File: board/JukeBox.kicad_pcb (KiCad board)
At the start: 2 copper layers, 88 x 88 mm, 68 parts, among them J1 USB_C_Receptacle_USB2.0, J2 Conn_01x03, J3 Conn_01x04, SW1 SW_SPST, SW10 SW_SPST, SW11 SW_SPST, SW12 SW_SPST, SW2 SW_SPST, SW3 SW_SPST, SW4 SW_SPST, SW5 SW_SPST, SW6 SW_SPST, SW7 SW_SPST, SW8 SW_SPST, SW9 SW_SPST, U1 NCP1117-3.3_SOT223, U2 W25Q128JVS, U3 RP2040, Y1 ABLS-12.000MHZ-B4-T

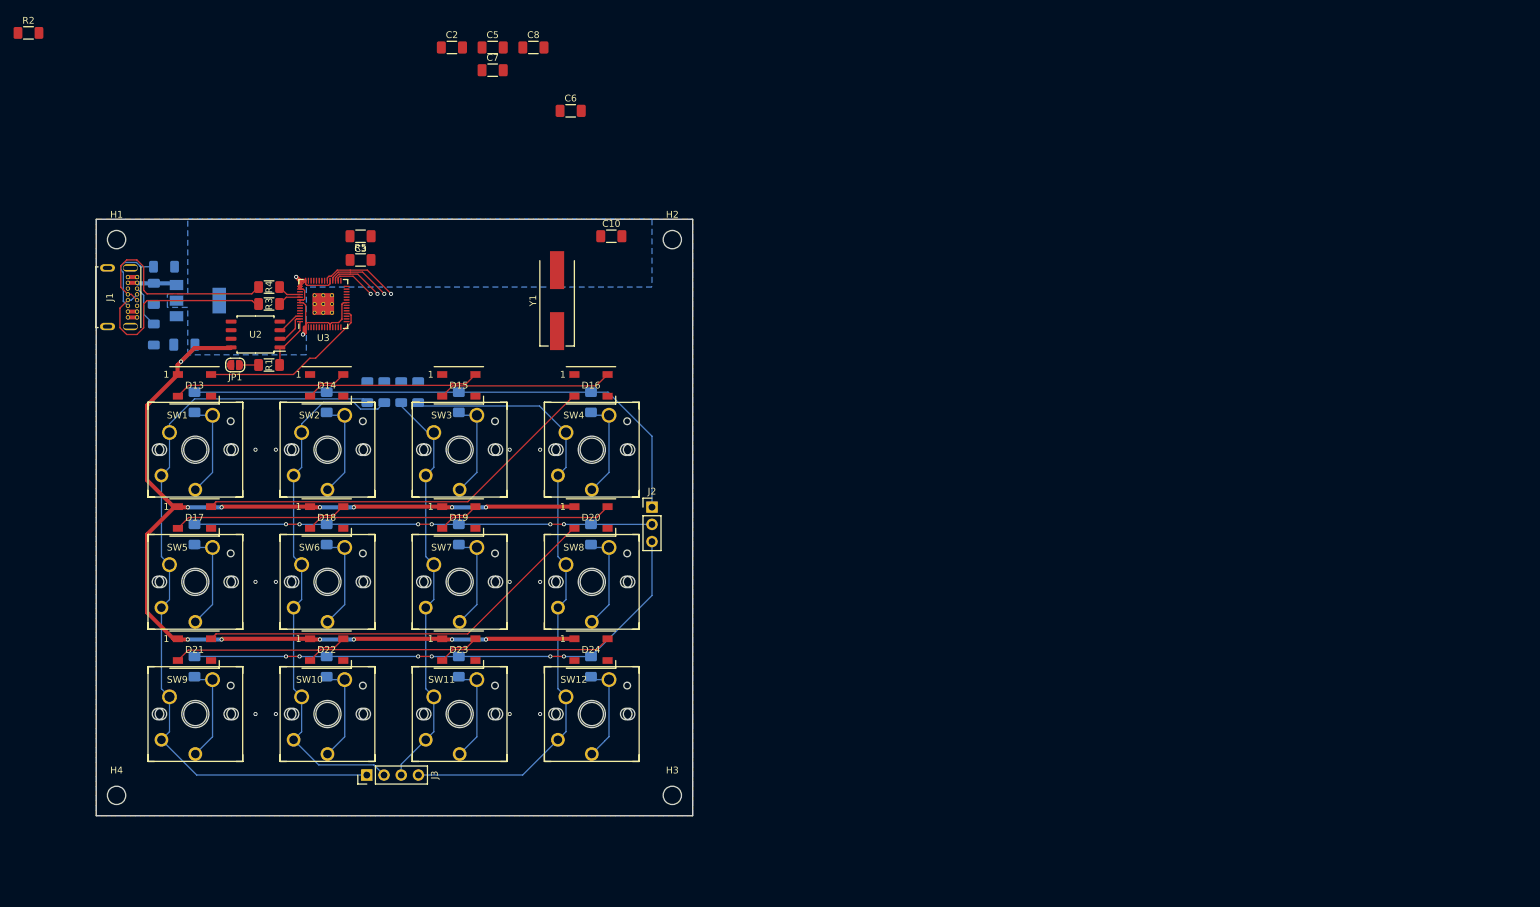
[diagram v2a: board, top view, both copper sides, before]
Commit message: second pass pcb
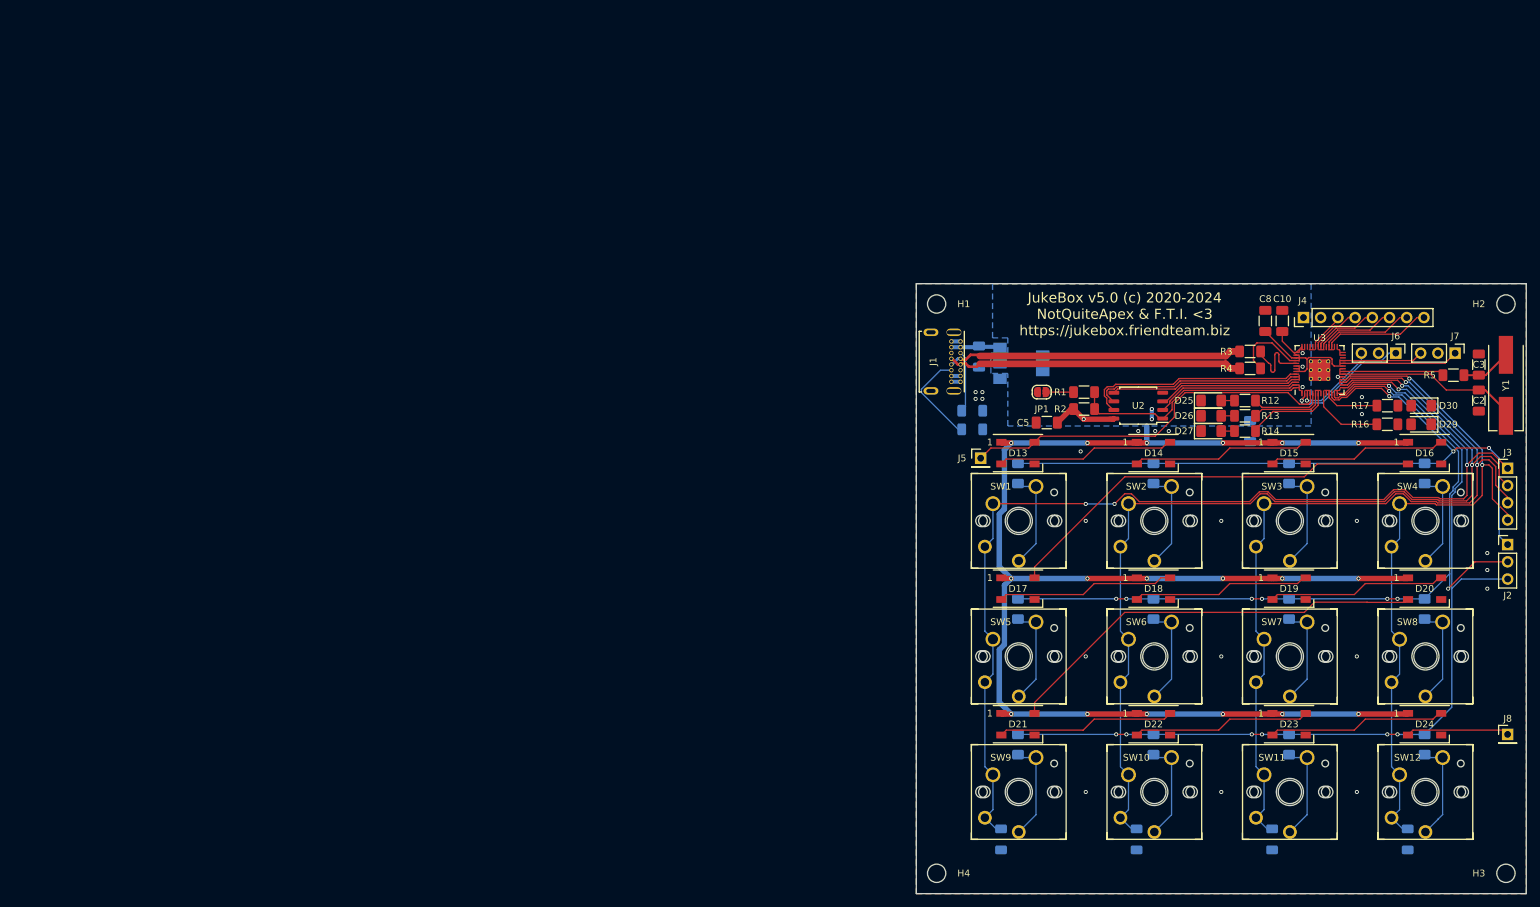
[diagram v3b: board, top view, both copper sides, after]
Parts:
- removed C6, C7: 100n, Capacitor_SMD:C_1206_3216Metric_Pad1.33x1.80mm_HandSolder
- added D25: LED, Diode_SMD:D_1206_3216Metric_Pad1.42x1.75mm_HandSolder, F.Cu at (211.1, 72.2)
- added D26: LED, Diode_SMD:D_1206_3216Metric_Pad1.42x1.75mm_HandSolder, F.Cu at (211.1, 74.5)
- added D27: LED, Diode_SMD:D_1206_3216Metric_Pad1.42x1.75mm_HandSolder, F.Cu at (211.1, 76.8)
- added D29: LED, Diode_SMD:D_1206_3216Metric_Pad1.42x1.75mm_HandSolder, F.Cu at (242.1, 75.8)
- added D30: LED, Diode_SMD:D_1206_3216Metric_Pad1.42x1.75mm_HandSolder, F.Cu at (242.1, 73.0)
- added J4: Conn_01x08, Connector_PinHeader_2.54mm:PinHeader_1x08_P2.54mm_Vertical, F.Cu at (224.7, 60.0)
- added J5: Conn_01x01, Connector_PinHeader_2.54mm:PinHeader_1x01_P2.54mm_Vertical, F.Cu at (177.1, 80.8)
- added J6: Conn_01x03, Connector_PinHeader_2.54mm:PinHeader_1x03_P2.54mm_Vertical, F.Cu at (238.3, 65.2)
- added J7: Conn_01x03, Connector_PinHeader_2.54mm:PinHeader_1x03_P2.54mm_Vertical, F.Cu at (247.1, 65.2)
- added J8: Conn_01x01, Connector_PinHeader_2.54mm:PinHeader_1x01_P2.54mm_Vertical, F.Cu at (254.8, 121.5)
- added R10: 10k, Resistor_SMD:R_1206_3216Metric_Pad1.30x1.75mm_HandSolder, B.Cu at (220.1, 137.0)
- added R16: 200, Resistor_SMD:R_1206_3216Metric_Pad1.30x1.75mm_HandSolder, F.Cu at (237.1, 75.8)
- added R17: 200, Resistor_SMD:R_1206_3216Metric_Pad1.30x1.75mm_HandSolder, F.Cu at (237.1, 73.0)
- added R8: 10k, Resistor_SMD:R_1206_3216Metric_Pad1.30x1.75mm_HandSolder, B.Cu at (180.1, 137.0)
- added R9: 10k, Resistor_SMD:R_1206_3216Metric_Pad1.30x1.75mm_HandSolder, B.Cu at (200.1, 137.0)
- R12, R13, R14: value 10k -> 200; moved to F.Cu
- moved J3 174.3 mm to (254.8, 82.2), turned to 0 degrees
- moved R11 167.1 mm to (240.1, 137.0), turned to 90 degrees
- moved C3 166.1 mm to (250.6, 66.9), turned to 90 degrees
- moved R2 165.3 mm to (192.3, 73.5)
- moved R5 162.1 mm to (246.8, 68.5)
- moved C2 160.2 mm to (250.6, 72.2), turned to -90 degrees
- moved C4 157.8 mm to (216.8, 76.8), turned to -90 degrees
- moved U3 147.3 mm to (227.1, 67.8)
- moved R4 145.2 mm to (216.8, 67.5)
- moved R3 144.9 mm to (216.8, 65.0)
- moved Y1 140.6 mm to (254.6, 70.0)
- moved U2 130.7 mm to (200.3, 73.0)
- moved R12 127.0 mm to (216.1, 72.2), turned to 180 degrees
- moved J2 126.4 mm to (254.8, 93.5)
- moved R13 124.5 mm to (216.1, 74.5), turned to 180 degrees
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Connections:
- net Net-(R3-Pad2) renamed /USB_R_D+
- net Net-(R4-Pad2) renamed /USB_R_D-
- D1 pad 1: /GPIO16 -> /GPIO9
- D10 pad 1: /GPIO18 -> /GPIO11
- D11 pad 1: /GPIO18 -> /GPIO11
- D12 pad 1: /GPIO18 -> /GPIO11
- D13 pad 4: /GPIO15 -> /GPIO2
- D2 pad 1: /GPIO16 -> /GPIO9
- D24 pad 2: unconnected-(D24-Pad2) -> /RGBDOUT
- D3 pad 1: /GPIO16 -> /GPIO9
- D4 pad 1: /GPIO16 -> /GPIO9
- D5 pad 1: /GPIO17 -> /GPIO10
- D6 pad 1: /GPIO17 -> /GPIO10
- D7 pad 1: /GPIO17 -> /GPIO10
- D8 pad 1: /GPIO17 -> /GPIO10
- D9 pad 1: /GPIO18 -> /GPIO11
- J1 pad P1: (no net) -> GND
- J1 pad P2: (no net) -> GND
- J1 pad P3: (no net) -> GND
- J1 pad P4: (no net) -> GND
- J2 pad 1: /GPIO16 -> /GPIO9
- J2 pad 2: /GPIO17 -> /GPIO10
- J2 pad 3: /GPIO18 -> /GPIO11
- J3 pad 1: /GPIO19 -> /GPIO12
- J3 pad 2: /GPIO20 -> /GPIO13
- J3 pad 3: /GPIO21 -> /GPIO14
- J3 pad 4: /GPIO22 -> /GPIO15
- R11 pad 2: /GPIO19 -> /GPIO15
- R12 pad 1: GND -> /GPIO3
- R12 pad 2: /GPIO20 -> Net-(R12-Pad2)
- R13 pad 1: GND -> /GPIO4
- R13 pad 2: /GPIO21 -> Net-(D26-Pad2)
- R14 pad 1: GND -> /GPIO5
- R14 pad 2: /GPIO22 -> Net-(D27-Pad2)
- SW1 pad 2: /GPIO19 -> /GPIO12
- SW10 pad 2: /GPIO20 -> /GPIO13
- SW11 pad 2: /GPIO21 -> /GPIO14
- SW12 pad 2: /GPIO22 -> /GPIO15
- SW2 pad 2: /GPIO20 -> /GPIO13
- SW3 pad 2: /GPIO21 -> /GPIO14
- SW4 pad 2: /GPIO22 -> /GPIO15
- SW5 pad 2: /GPIO19 -> /GPIO12
- SW6 pad 2: /GPIO20 -> /GPIO13
- SW7 pad 2: /GPIO21 -> /GPIO14
- SW8 pad 2: /GPIO22 -> /GPIO15
- SW9 pad 2: /GPIO19 -> /GPIO12
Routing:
- net /GPIO12: track 0.00 -> 162.6 mm, vias 0 -> 4
- net /GPIO13: track 0.00 -> 144.2 mm, vias 0 -> 2
- net /GPIO11: track 0.00 -> 136.1 mm, vias 0 -> 7
- net /GPIO14: track 0.00 -> 125.6 mm, vias 0 -> 2
- net /GPIO10: track 0.00 -> 120.1 mm, vias 0 -> 8
- net /GPIO19: track 118.9 -> 0.00 mm, vias 1 -> 0
- net /GPIO9: track 0.00 -> 109.1 mm, vias 0 -> 3
- net /GPIO22: track 105.9 -> 11.8 mm, vias 1 -> 0
- net /GPIO15: track 25.7 -> 107.0 mm, vias 0 -> 2
- net /GPIO16: track 80.7 -> 0.00 mm
- net /GPIO18: track 79.2 -> 0.00 mm, vias 6 -> 0
- net /GPIO20: track 87.0 -> 15.8 mm, vias 1 -> 0
- net /GPIO17: track 67.5 -> 0.00 mm, vias 6 -> 0
- net /GPIO21: track 71.2 -> 13.7 mm, vias 1 -> 0
- net /GPIO2: track 0.00 -> 56.0 mm
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- added copper zone on F.Cu, net +3V3
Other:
- board size 88 x 88 mm -> 90 x 90 mm
- board text added: "JukeBox v5.0 (c) 2020-2024 NotQuiteApex & F.T.I. <3 https://jukebox.friendteam.biz"
